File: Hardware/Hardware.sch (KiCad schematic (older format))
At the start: 12 parts

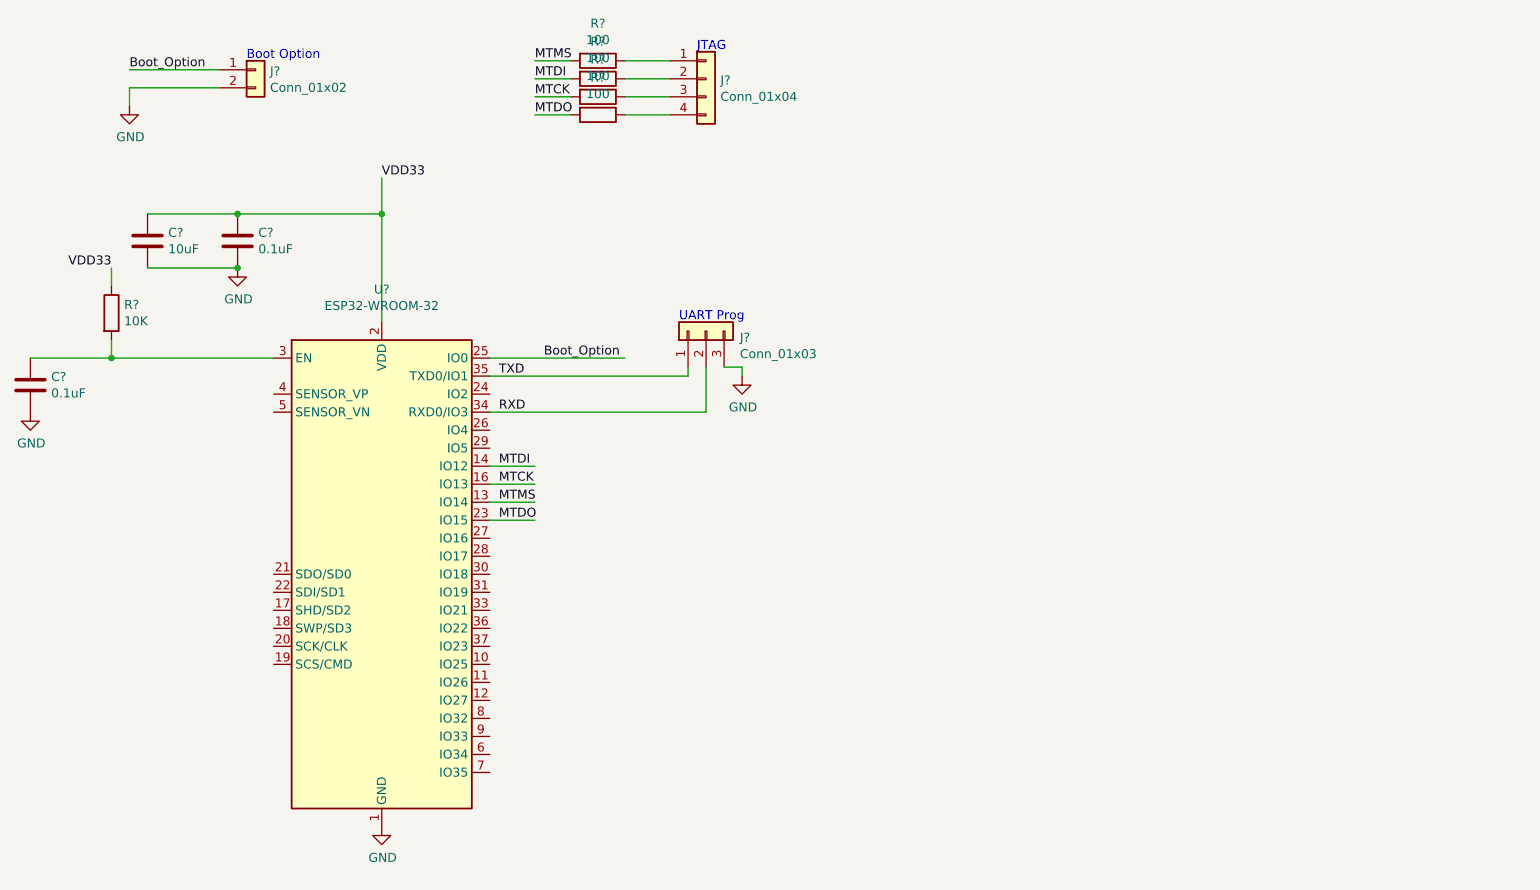
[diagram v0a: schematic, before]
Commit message: Hardware dev
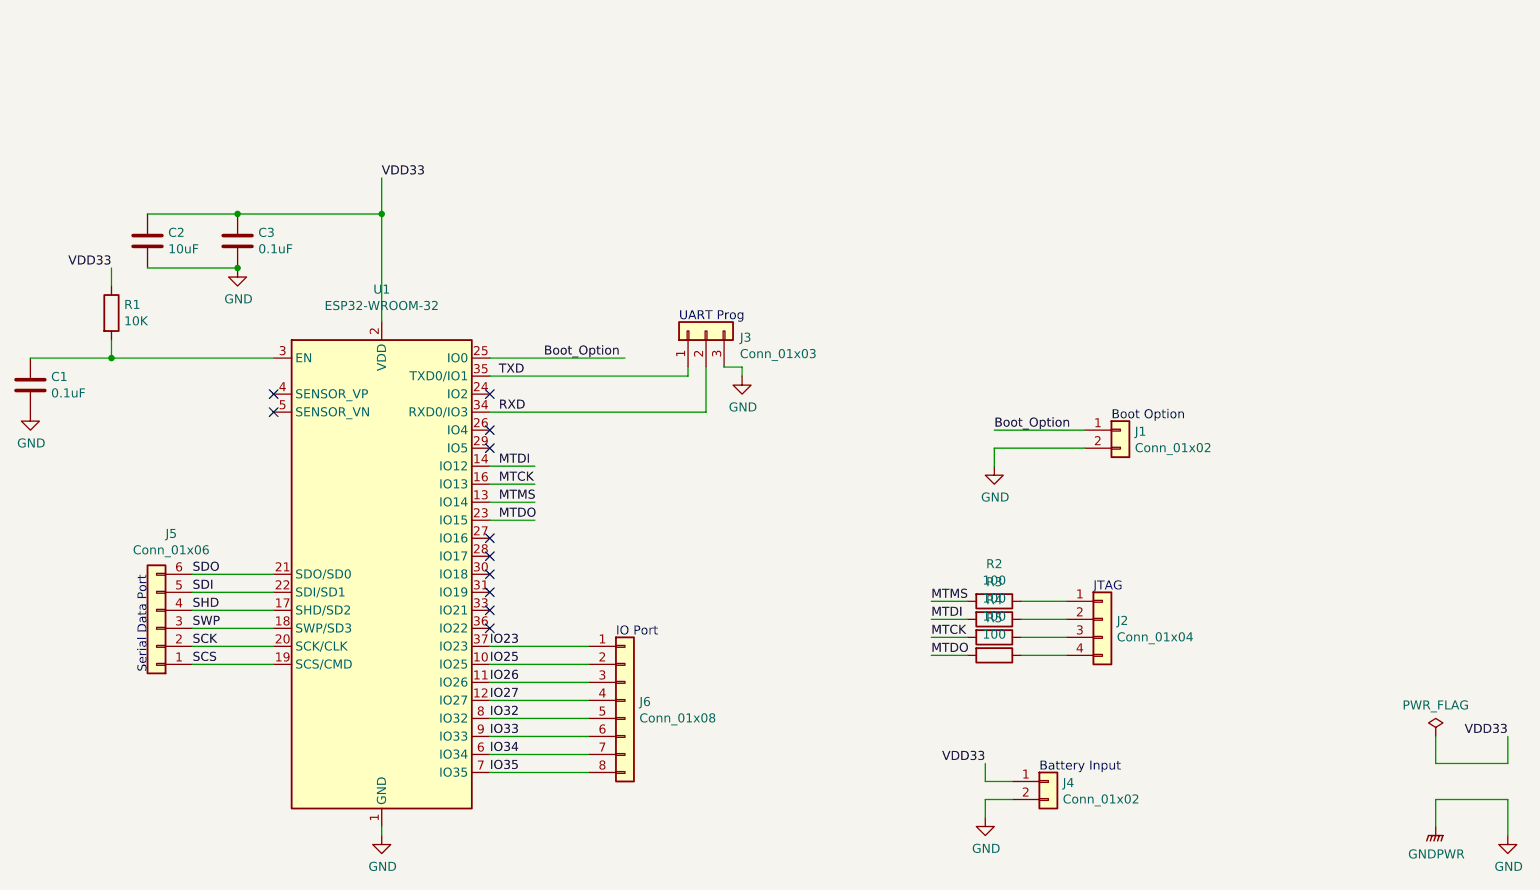
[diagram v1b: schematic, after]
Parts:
- added J4: Conn_01x02, Connector_PinHeader_2.54mm:PinHeader_1x02_P2.54mm_Vertical, symbol Connector_Generic:Conn_01x02
- added J5: Conn_01x06, Connector_PinHeader_2.54mm:PinHeader_1x06_P2.54mm_Vertical, symbol Connector_Generic:Conn_01x06
- added J6: Conn_01x08, Connector_PinHeader_2.54mm:PinHeader_1x08_P2.54mm_Vertical, symbol Connector_Generic:Conn_01x08
- C1, C2, C3: renamed from C?; footprint (none) -> Connector_PinHeader_2.54mm:PinHeader_1x02_P2.54mm_Vertical
- J1: renamed from J?; footprint (none) -> Connector_PinHeader_2.54mm:PinHeader_1x02_P2.54mm_Vertical
- J2: renamed from J?; footprint (none) -> Connector_PinHeader_2.54mm:PinHeader_1x04_P2.54mm_Vertical
- J3: renamed from J?; footprint (none) -> Connector_PinHeader_2.54mm:PinHeader_1x03_P2.54mm_Vertical
- R1, R2, R3, R4, R5: renamed from R?; footprint (none) -> Connector_PinHeader_2.54mm:PinHeader_1x02_P2.54mm_Vertical
- gave numbers to parts that had none: 1
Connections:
- net labels added: GNDPWR, IO23, IO25, IO26, IO27, IO32, IO33, IO34, IO35, SCK, SCS, SDI, SDO, SHD, SWP
- wire segments 31 -> 56
- no-connect marks 0 -> 11
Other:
- note added: "Battery Input"
- note added: "IO Port"
- note added: "Serial Data Port"
- moved on the sheet: J1, J2, R2, R3, R4, R5
